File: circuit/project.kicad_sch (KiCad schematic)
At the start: 0 parts

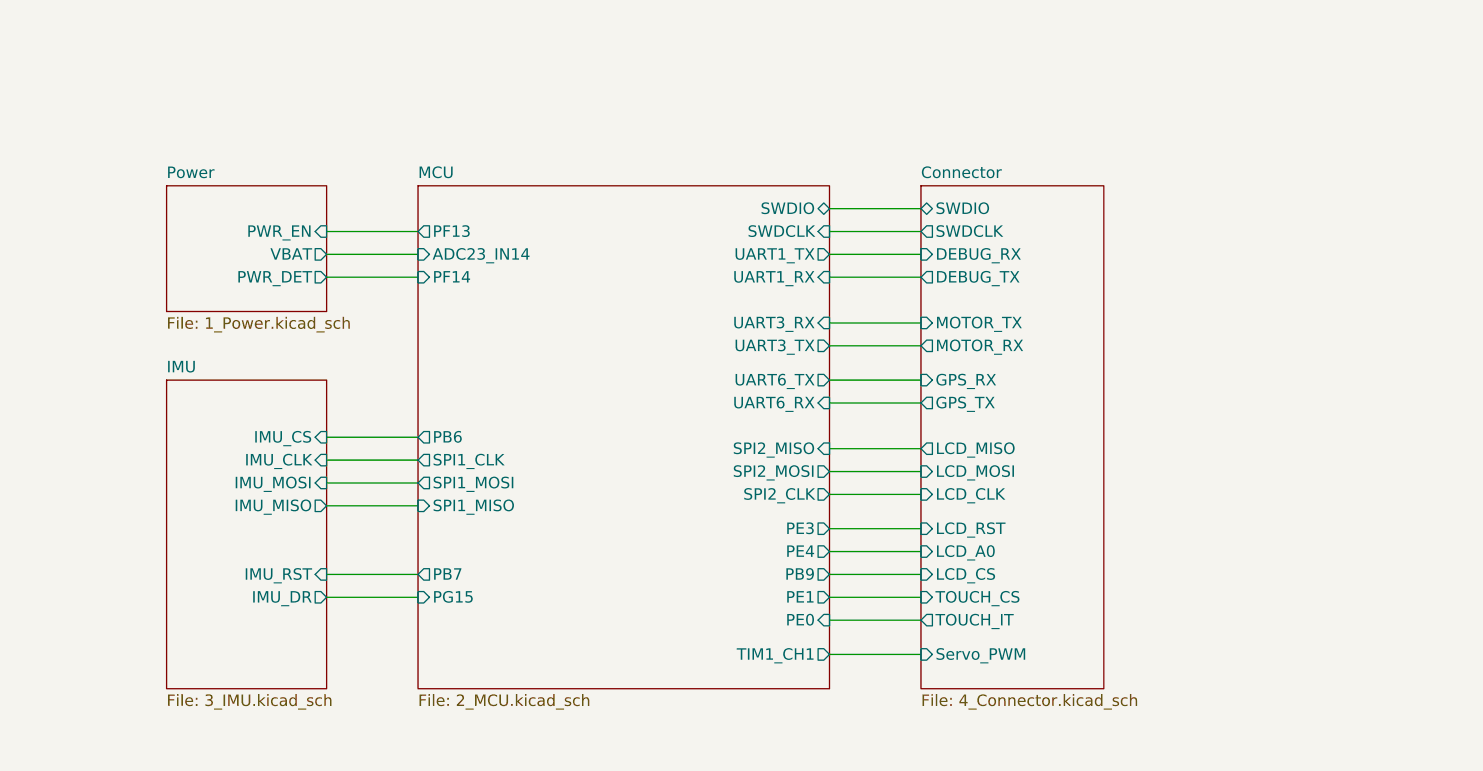
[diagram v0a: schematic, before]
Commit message: Update circuit with control mcu.
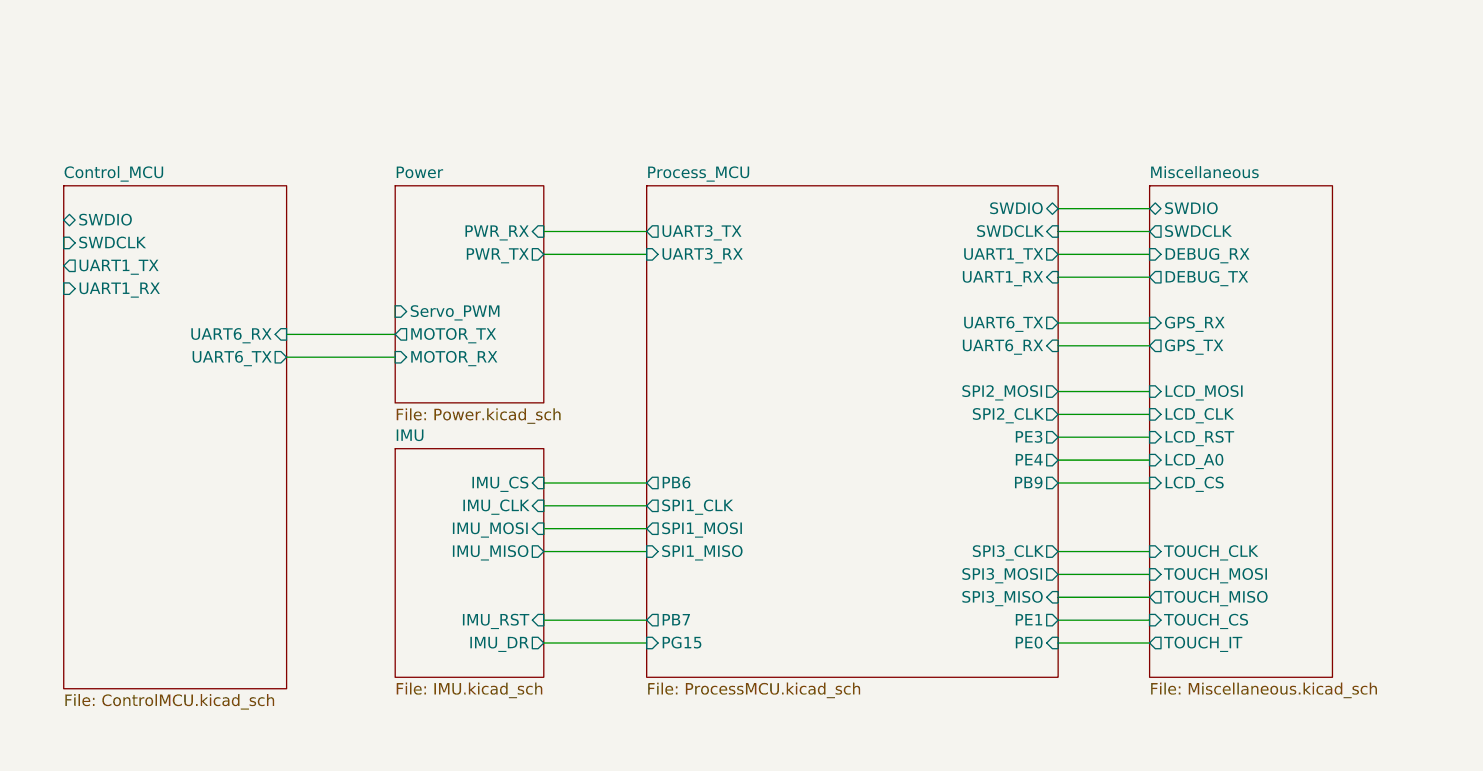
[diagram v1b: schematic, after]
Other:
- sheet Connector renamed Miscellaneous
- sheet MCU renamed Process_MCU
- added sheet Control_MCU (ControlMCU.kicad_sch)
- sheet IMU: file 3_IMU.kicad_sch -> IMU.kicad_sch
- sheet Miscellaneous: file 4_Connector.kicad_sch -> Miscellaneous.kicad_sch
- sheet Miscellaneous ports: added TOUCH_CLK, TOUCH_MISO, TOUCH_MOSI; removed LCD_MISO, MOTOR_RX, MOTOR_TX, Servo_PWM
- sheet Power: file 1_Power.kicad_sch -> Power.kicad_sch
- sheet Power ports: added MOTOR_RX, MOTOR_TX, PWR_RX, PWR_TX, Servo_PWM; removed PWR_DET, PWR_EN, VBAT
- sheet Process_MCU: file 2_MCU.kicad_sch -> ProcessMCU.kicad_sch
- sheet Process_MCU ports: added SPI3_CLK, SPI3_MISO, SPI3_MOSI; removed ADC23_IN14, PF13, PF14, SPI2_MISO, TIM1_CH1

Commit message: Update circuit and ADIS16470 footprint reference datasheet.
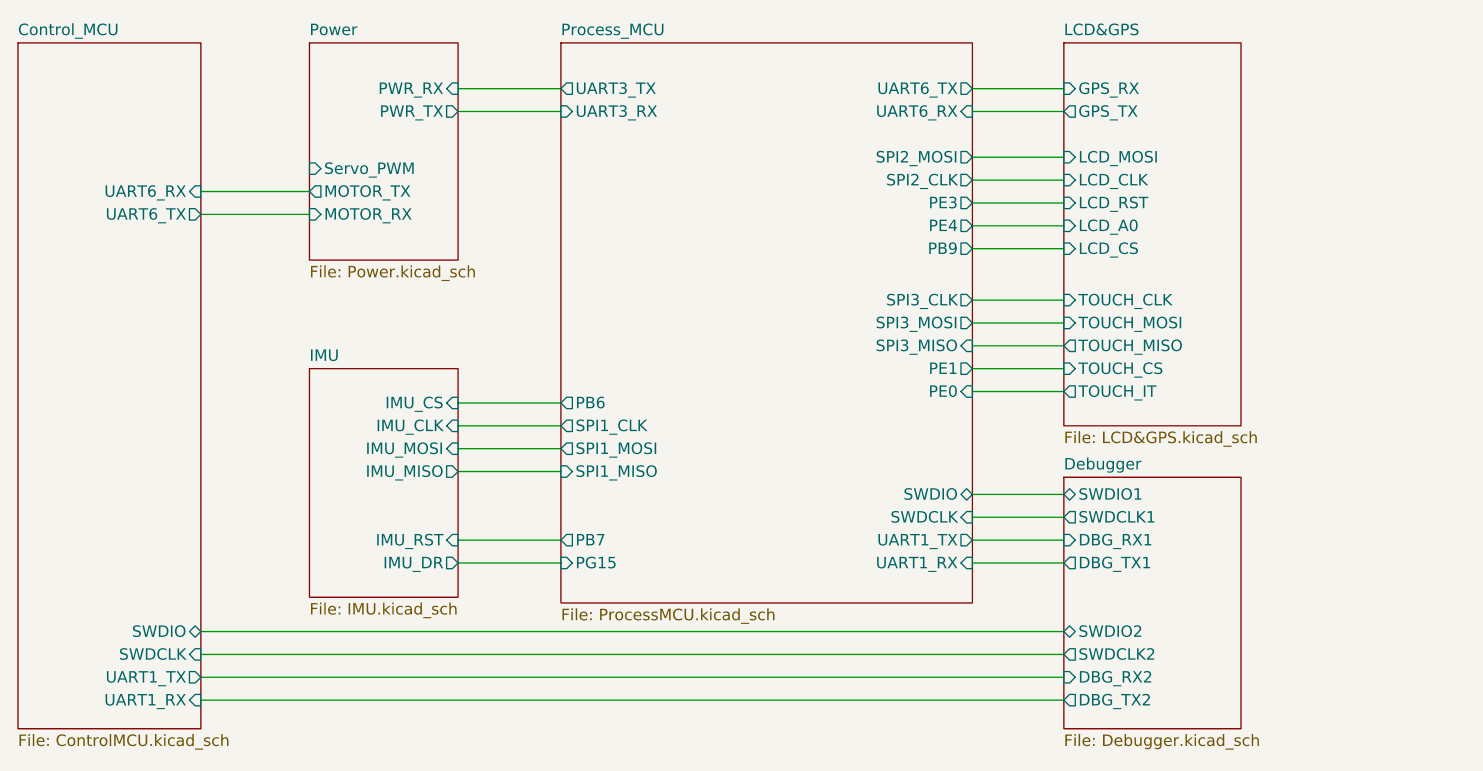
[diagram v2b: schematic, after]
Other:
- sheet Miscellaneous renamed LCD&GPS
- added sheet Debugger (Debugger.kicad_sch)
- sheet LCD&GPS: file Miscellaneous.kicad_sch -> LCD&GPS.kicad_sch
- sheet LCD&GPS ports: added none; removed DEBUG_RX, DEBUG_TX, SWDCLK, SWDIO
